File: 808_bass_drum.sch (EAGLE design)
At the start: 56 parts, among them IC1 TL072P, Q1 2N3906, Q10 2N3904, Q11 2N3904, Q7 2N3904, Q8 2N3904, Q9 2N3904

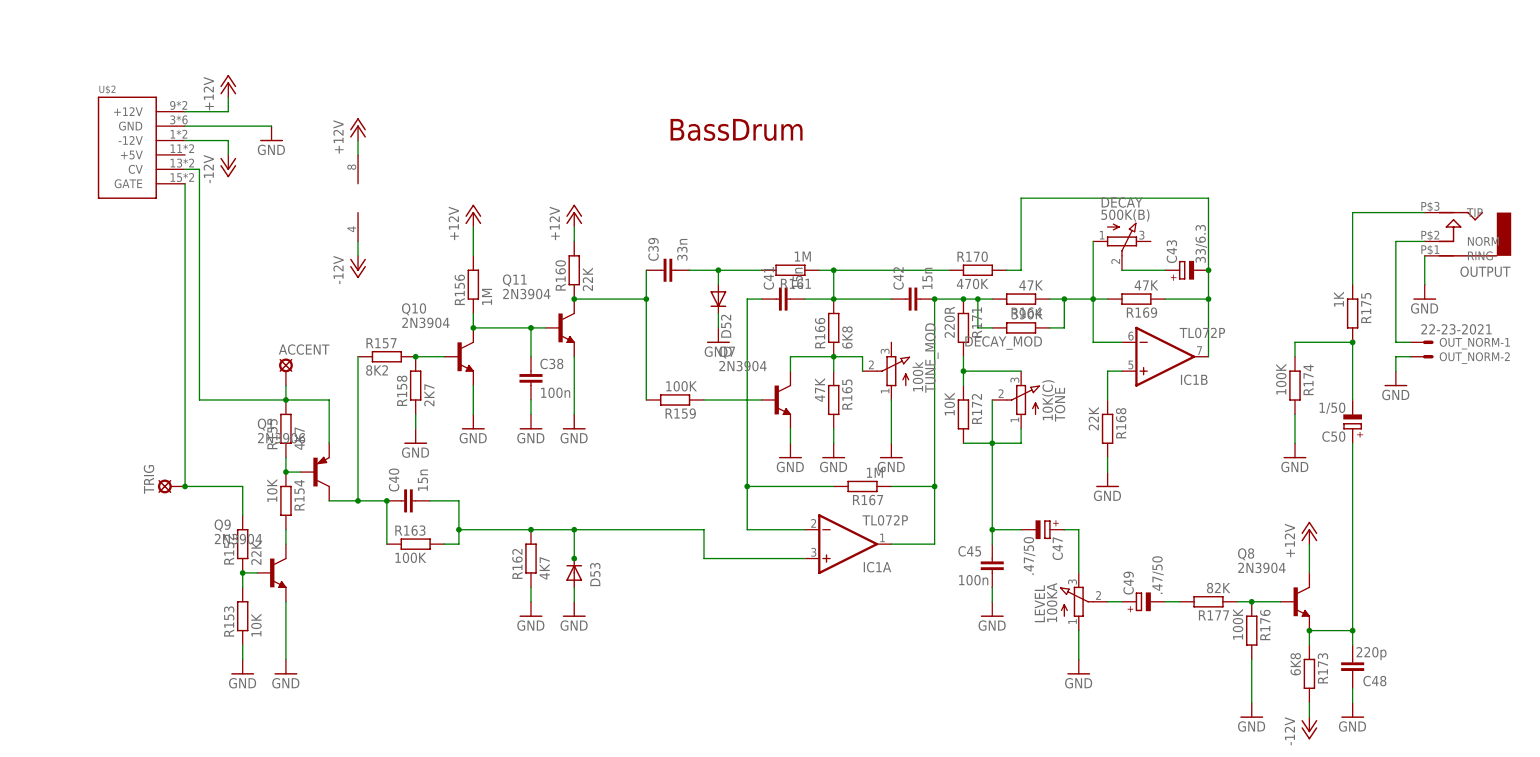
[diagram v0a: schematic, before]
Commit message: 93pct ar
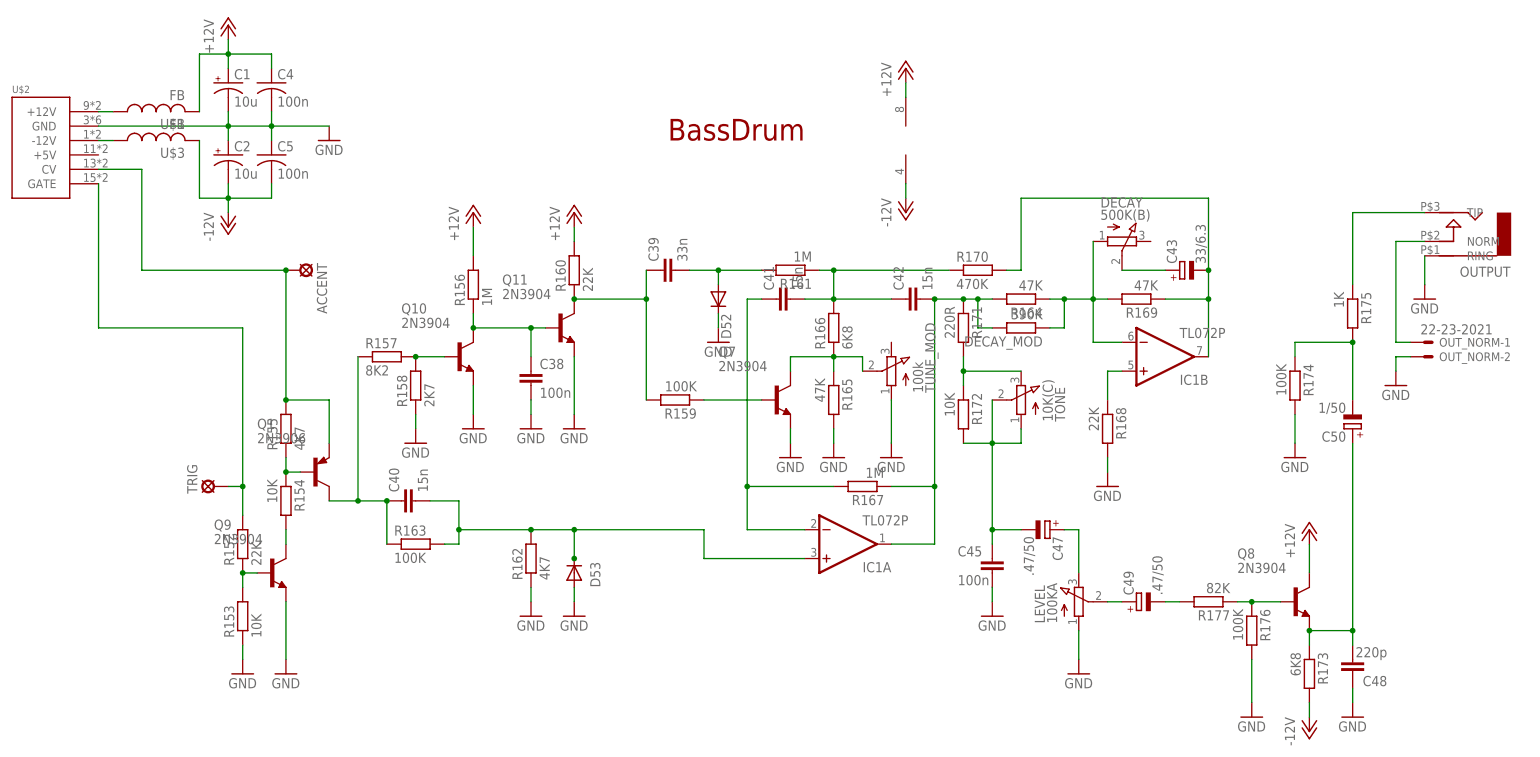
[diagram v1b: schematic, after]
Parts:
- added C1, C2: 10u, rcl:CPOL-USB45181A
- added C4, C5: 100n, rcl:C-US050-024X044
- added U$1, U$3: FB, adafruit:FB
- C38, C45: device TR808clone:C-EU075-032X103 -> TR808clone:C-EU050-030X075
- C39: device TR808clone:C-EU050-024X044 -> TR808clone:C-EU050-025X075
- C48: device TR808clone:C-EU025-025X050 -> TR808clone:C-EU050-025X075
- R156, R159, R160, R161, R165, R167, R168, R169, R171, R174, R177: device TR808clone:R-EU_0207/5V -> TR808clone:R-EU_0207/7
- R166, R173, R175, R176: device TR808clone:R-EU_0207/5V -> TR808clone:R-EU_0309/10
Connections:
- new net N$5: U$1.1, U$2.+12V
- new net N$6: U$2.-12V, U$3.1
- net +12V: now also C1.+, C4.1, U$1.2; no longer U$2.+12V
- net -12V: now also C2.-, C5.2, U$3.2; no longer U$2.-12V
- net GND: now also C1.-, C2.+, C4.2, C5.1
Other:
- moved on the sheet: ACCENT, TRIG, U$2
